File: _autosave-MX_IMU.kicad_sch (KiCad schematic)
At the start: 24 parts, among them U1 STM32F405RGT6, Y1 16MHz

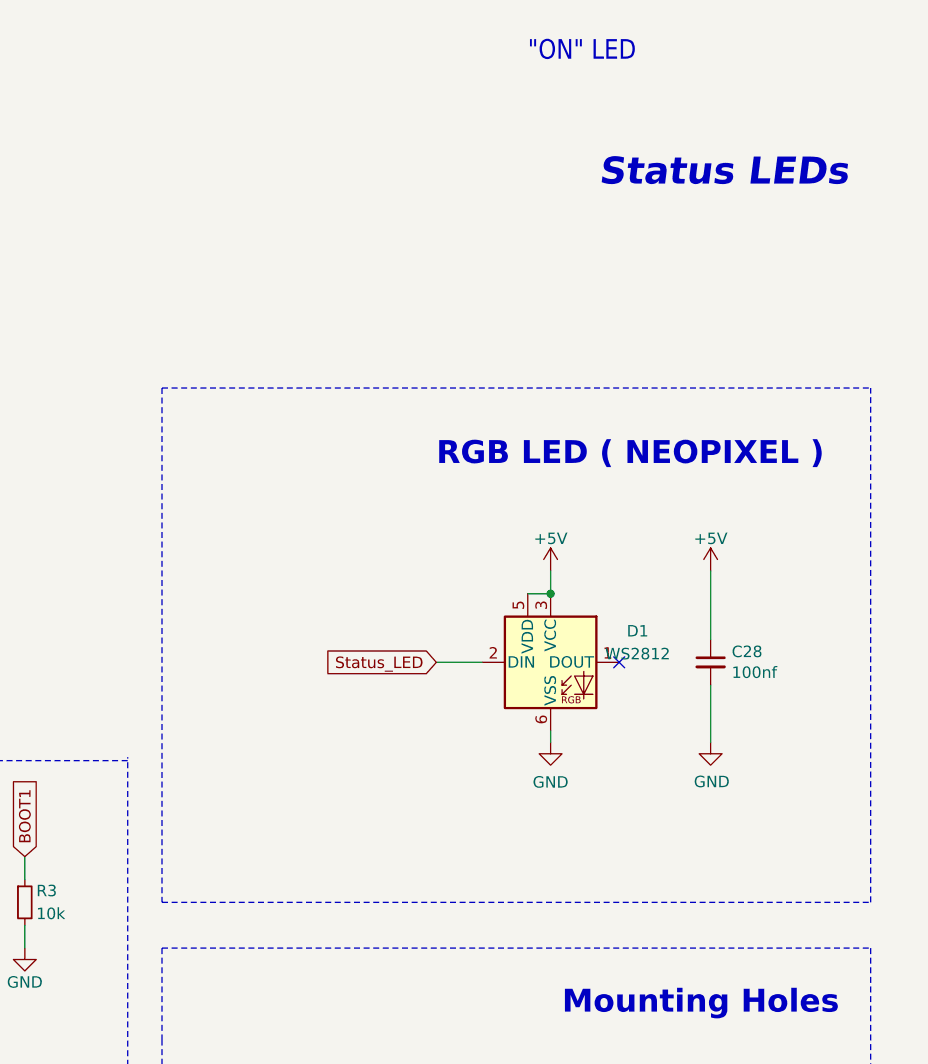
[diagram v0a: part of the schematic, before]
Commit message: update
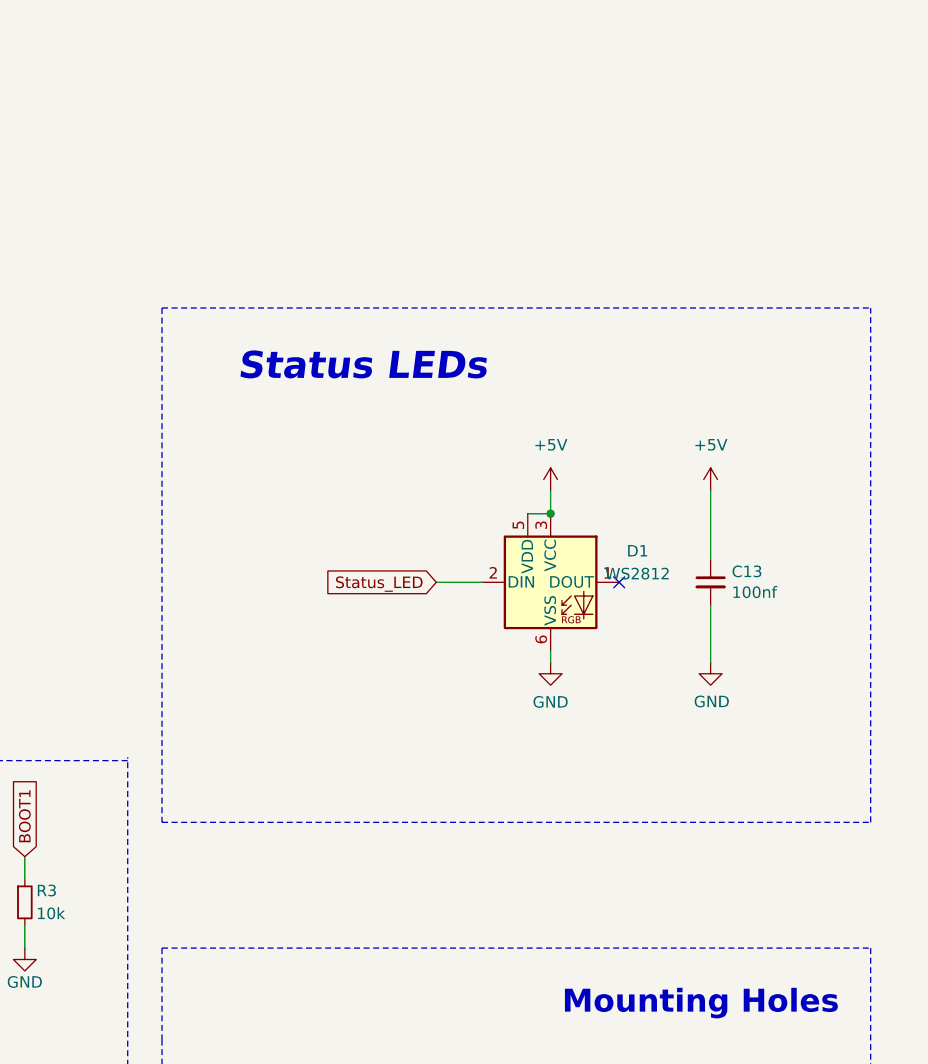
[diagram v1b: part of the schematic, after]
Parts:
- renumbered C28 to C13
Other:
- note removed: ""ON" LED"
- note removed: "RGB LED ( NEOPIXEL )"
- moved on the sheet: C13, D1
